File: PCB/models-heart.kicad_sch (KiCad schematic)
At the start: 103 parts, among them P1 USB_C_Plug, Q1 AO3401A, Q2 FS8205, Q3 UMH3N, Q4 AO3401A, Q5 AO3401A, Q6 BC857BS, Q7 BC857BS, Q8 AO3401A, Q9 UMH3N, SW1 SW_Push, U1 TP4056, U2 DW01, U3 CH340C, U4 AMS1117-3.3, U5 ESP-12E, U6 DRV8833PWP

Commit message: PCB Done
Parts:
- C14: footprint Capacitor_SMD:C_1206_3216Metric -> Capacitor_SMD:C_0805_2012Metric
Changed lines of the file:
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@@
       (effects (font (size 1.27 1.27)) (justify left))
     )
-    (property "Footprint" "Capacitor_SMD:C_1206_3216Metric" (at 268.9352 213.36 0)
+    (property "Footprint" "Capacitor_SMD:C_0805_2012Metric" (at 268.9352 213.36 0)
       (effects (font (size 1.27 1.27)) hide)
     )

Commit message: Production
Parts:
- C1, C10, C13, C2, C4, C5, C6: LCSC (none) -> C13585
- C11, C12, C3, C7, C8, C9: LCSC (none) -> C913910
- C14: LCSC (none) -> C49217
- D1: LCSC (none) -> C2286
- D2: LCSC (none) -> C2290
- P1: LCSC (none) -> C2927038
- Q1, Q4, Q5, Q8: LCSC (none) -> C15127
- Q2: LCSC (none) -> C908265
- Q3, Q9: LCSC (none) -> C62892
- Q6, Q7: LCSC (none) -> C699266
- R1, R10, R2: LCSC (none) -> C21190
- R11, R12, R13, R14, R21, R25: LCSC (none) -> C25803
- R15, R16, R17, R18, R19, R22, R24, R4, R7, R8: LCSC (none) -> C25804
- R20, R23: LCSC (none) -> C22961
- R3: LCSC (none) -> C22775
- R5, R6: LCSC (none) -> C23179
- U1: LCSC (none) -> C16581
- U2: LCSC (none) -> C917079
- U3: LCSC (none) -> C84681
- U4: LCSC (none) -> C880752
- U5: LCSC (none) -> C89297
- U6: LCSC (none) -> C50506

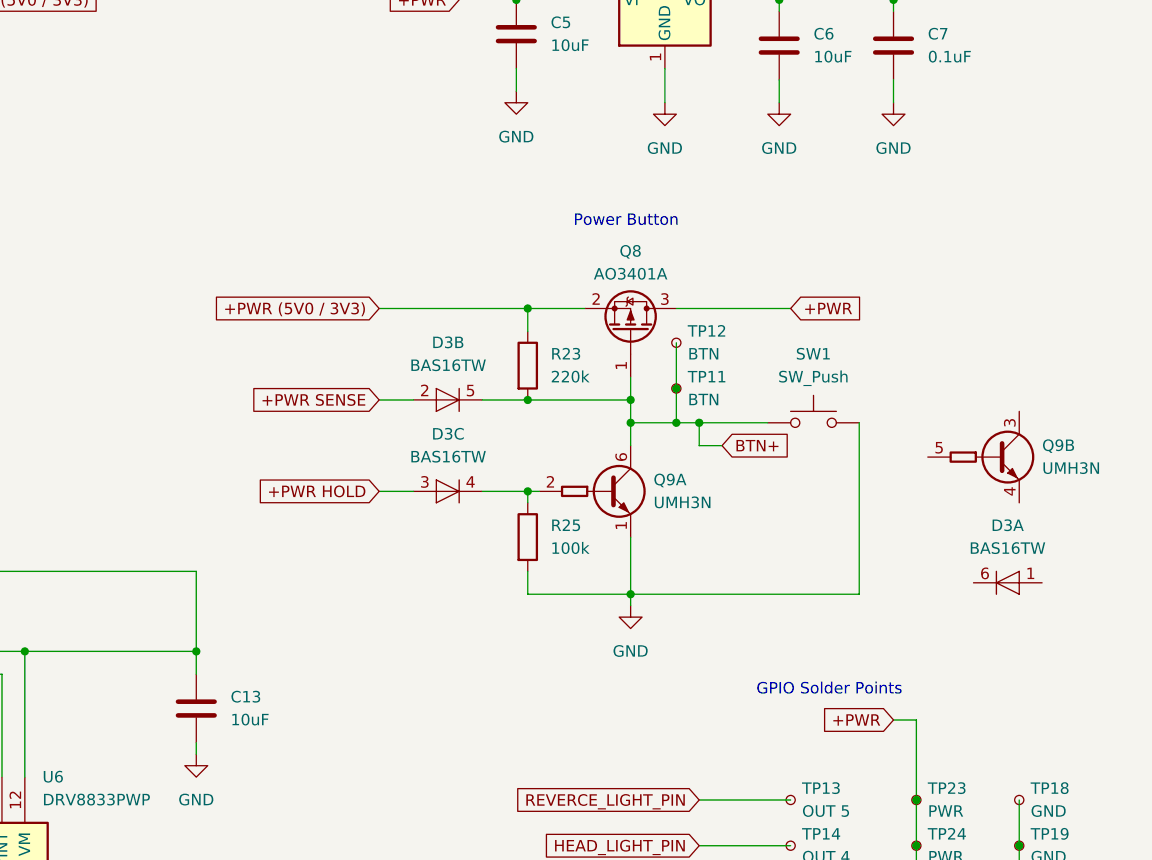
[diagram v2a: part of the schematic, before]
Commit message: Fabrication
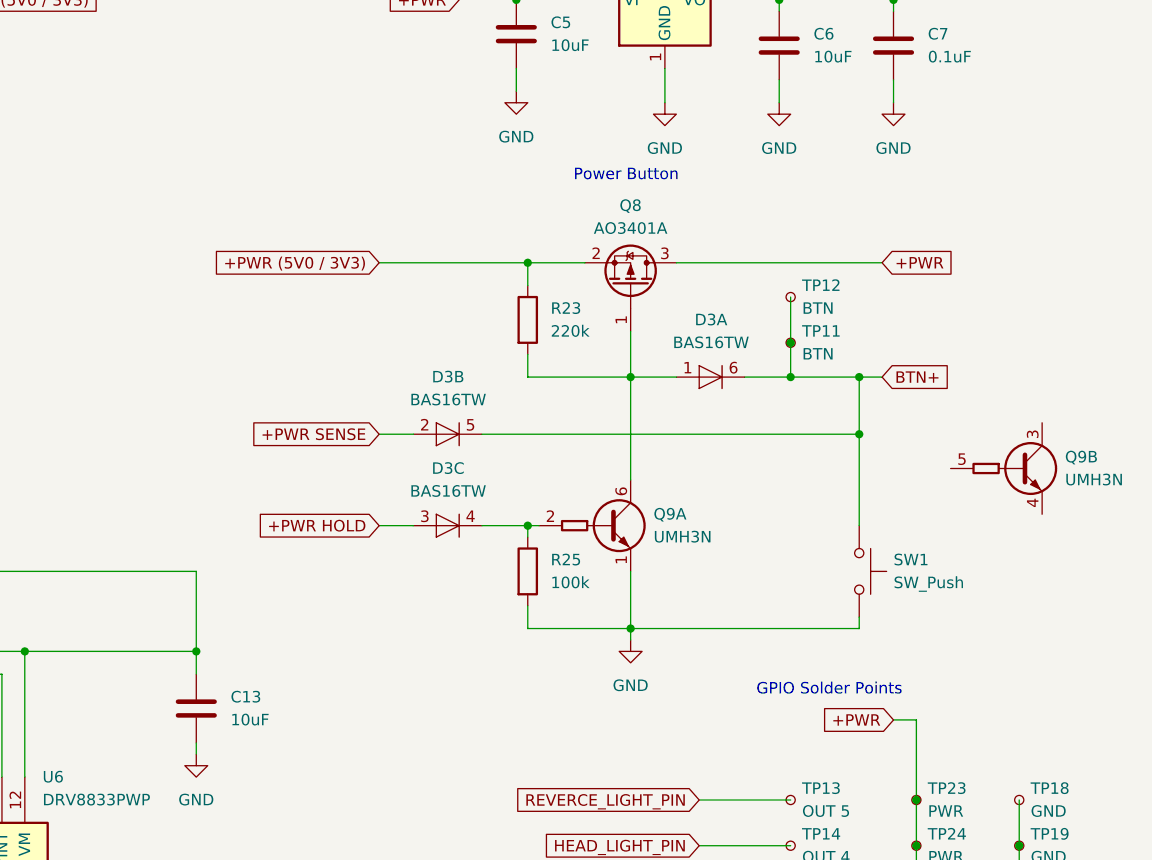
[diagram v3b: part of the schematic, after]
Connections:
- net BTN+: now also D3.6 (K); no longer Q8.1 (G), Q9.6 (C1), R23.2
- net at D3.1 (A): now also Q8.1 (G), Q9.6 (C1), R23.2
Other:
- moved on the sheet: D3A, D3B, D3C, Q8, Q9A, Q9B, R23, R25, SW1, TP11, TP12
